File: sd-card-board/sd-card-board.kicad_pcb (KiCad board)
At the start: 2 copper layers, 22.9 x 19.1 mm, 9 parts, among them J1 Conn_01x08, J2 Conn_01x02, J3 1051620001, U1 MIC5365-3.3YC5-TR, U2 FXMAR2104UMX

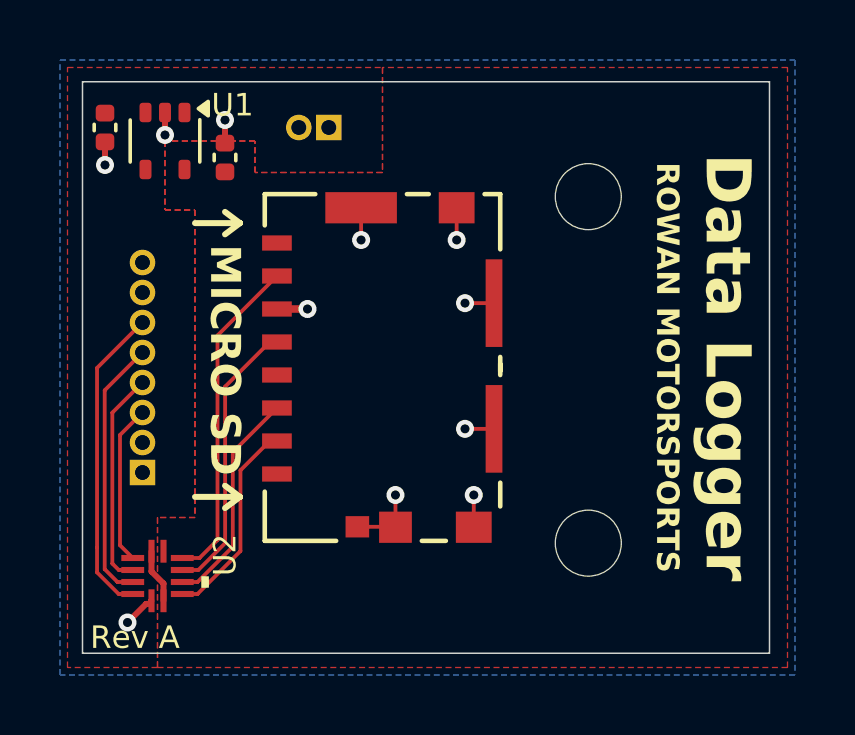
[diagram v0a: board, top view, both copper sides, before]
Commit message: sd-card-board: Fully fix positioning issues
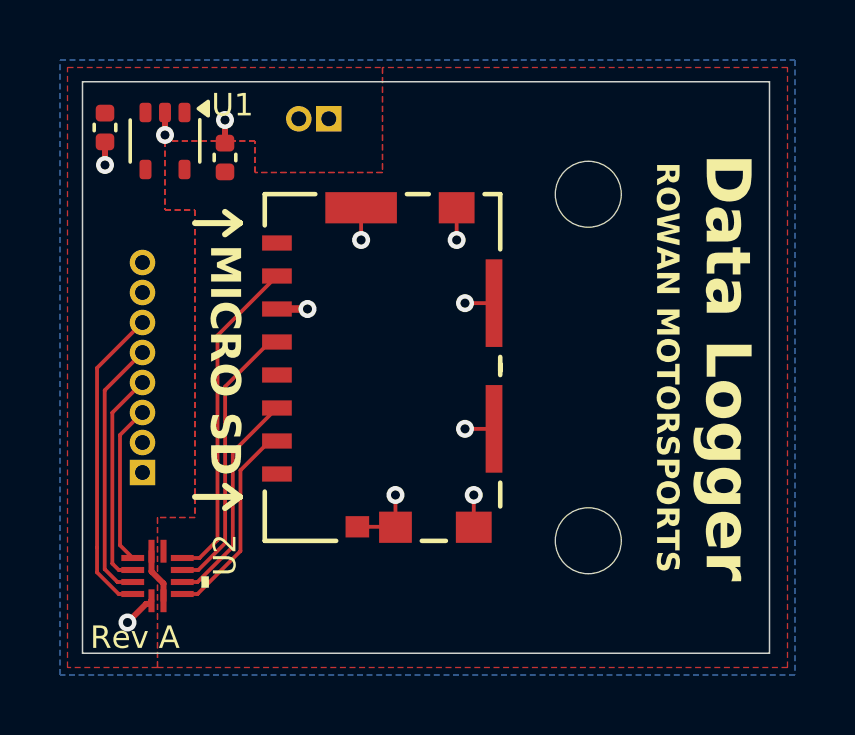
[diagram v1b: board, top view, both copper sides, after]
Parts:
- moved J2 0.29 mm to (112.0, 73.0)
- moved REF** 0.08 mm to (120.6, 75.5)
- moved REF** 0.08 mm to (120.6, 87.0)
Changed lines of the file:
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@@
 	(footprint "MountingHole:MountingHole_2.2mm_M2"
 		(layer "F.Cu")
-		(at 120.61 87.105)
+		(at 120.61 87.025)
 		(descr "Mounting Hole 2.2mm, M2, no annular, generated by kicad-footprint-generator mountinghole.py")
 		(tags "mountinghole M2")
@@
 	(footprint "MountingHole:MountingHole_2.2mm_M2"
 		(layer "F.Cu")
-		(at 120.61 75.555)
+		(at 120.61 75.475)
 		(descr "Mounting Hole 2.2mm, M2, no annular, generated by kicad-footprint-generator mountinghole.py")
 		(tags "mountinghole M2")
@@
 	(footprint "Connector_PinSocket_1.00mm:PinSocket_1x02_P1.00mm_Vertical"
 		(layer "B.Cu")
-		(at 111.96 73.25 90)
+		(at 111.96 72.96 90)
 		(descr "Through hole straight socket strip, 1x02, 1.00mm pitch, single row (https://gct.co/files/drawings/bc065.pdf), script generated")
 		(tags "Through hole socket strip THT 1x02 1.00mm single row")
@@
 		(layer "F.Fab")
 		(pts
-			(xy 105.75 77.75) (xy 111.25 73.25)
+			(xy 105.75 77.75) (xy 109.71 73.25)
 		)
 		(height -2.25)
@@
 			(thickness 0.1)
 			(arrow_length 1.27)
-			(text_position_mode 0)
+			(text_position_mode 2)
 			(arrow_direction outward)
 			(extension_height 0.58642)
@@
 		)
 		(gr_text "4.5"
-			(at 102.35 75.5 90)
+			(at 100.5 75.249998 90)
 			(layer "F.Fab")
 			(effects
@@
 		(layer "F.Fab")
 		(pts
-			(xy 120.9 75.555) (xy 120.9 87.105)
+			(xy 120.61 75.475) (xy 120.61 87.025)
 		)
 		(height -20.9)
@@
 		)
 		(gr_text "11.55"
-			(at 98.85 81.33 90)
+			(at 98.56 81.25 90)
 			(layer "F.Fab")
 			(effects
@@
 			(layer "F.Fab")
 			(effects
+				(font
+					(size 1 1)
+					(thickness 0.15)
+				)
+			)
+		)
+	)
+	(dimension
+		(type orthogonal)
+		(layer "F.Fab")
+		(pts
+			(xy 113.21 73.25) (xy 120.61 75.475)
+		)
+		(height -17.46)
+		(orientation 1)
+		(format
+			(prefix "")
+			(suffix "")
+			(units 3)
+			(units_format 0)
+			(precision 4)
+			(suppress_zeroes yes)
+		)
+		(style
+			(thickness 0.1)
+			(arrow_length 1.27)
+			(text_position_mode 0)
+			(arrow_direction outward)
+			(extension_height 0.58642)
+			(extension_offset 0.5)
+			(keep_text_aligned yes)
+		)
+		(gr_text "2.225"
+			(at 94.6 74.3625 90)
+			(layer "F.Fab")
+			(effects
